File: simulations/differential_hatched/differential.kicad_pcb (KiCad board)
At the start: 2 copper layers, 1.3 x 3.1 mm, 5 parts

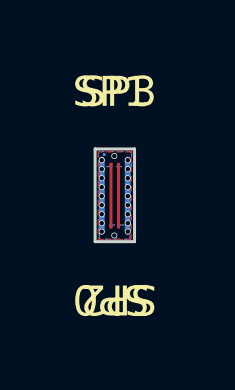
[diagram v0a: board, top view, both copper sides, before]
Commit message: Updated trace width to 0.15mm instead of 0.1mm
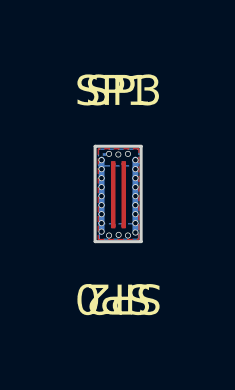
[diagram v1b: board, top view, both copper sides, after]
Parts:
- SP0, SP1, SP2, SP3: footprint simulation_port:pad_0.1mm -> simulation_port:pad_0.15mm
- moved SP2 0.18 mm to (148.9, 126.4)
- moved SP3 0.18 mm to (148.9, 128.5)
- moved SP0 0.08 mm to (148.6, 126.4)
- moved SP1 0.08 mm to (148.6, 128.5)
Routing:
- net GND: vias 20 -> 24
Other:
- board size 1.3 x 3.1 mm -> 1.5 x 3.2 mm
